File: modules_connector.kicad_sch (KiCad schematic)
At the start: 26 parts, among them J3 Conn_01x03, J4 Conn_01x03, J5 Conn_01x03, J9 Conn_01x04, K1 HE721A0500, K2 HE721A0500, Q1 BC847, Q2 BC847

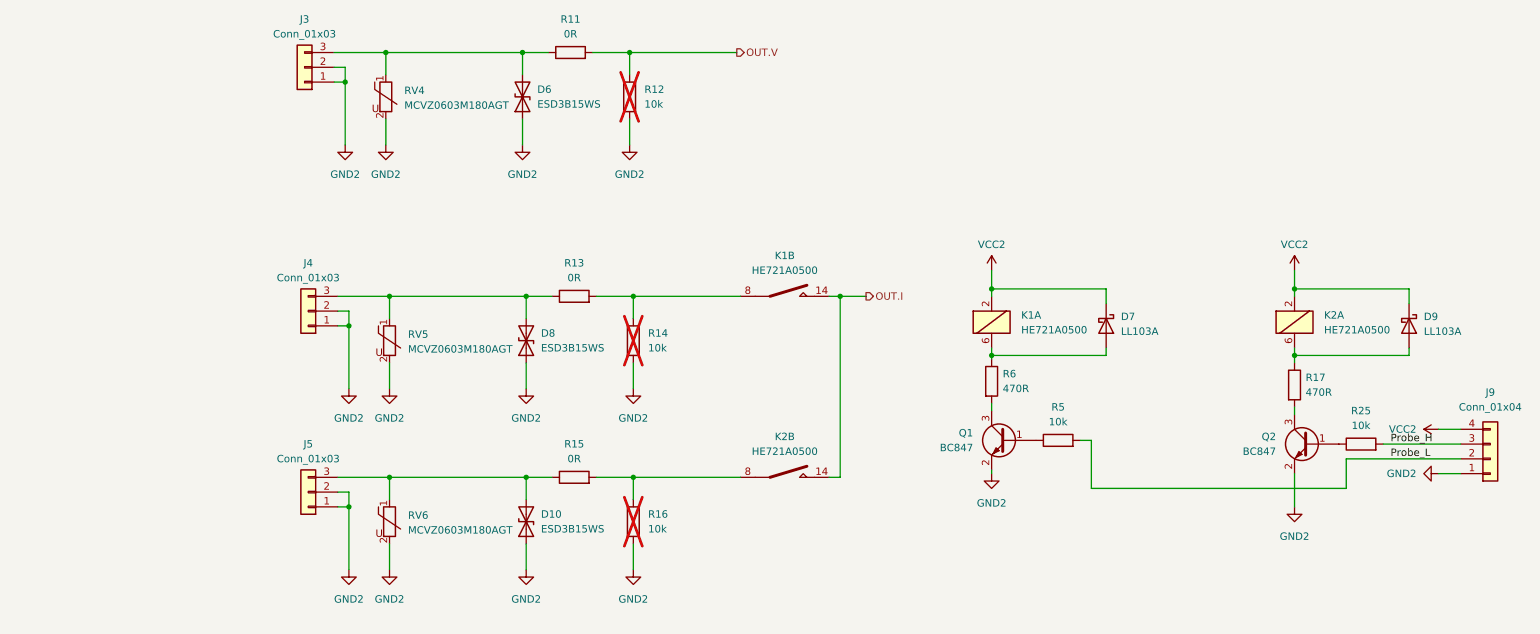
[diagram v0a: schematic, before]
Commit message: Redesign pcb
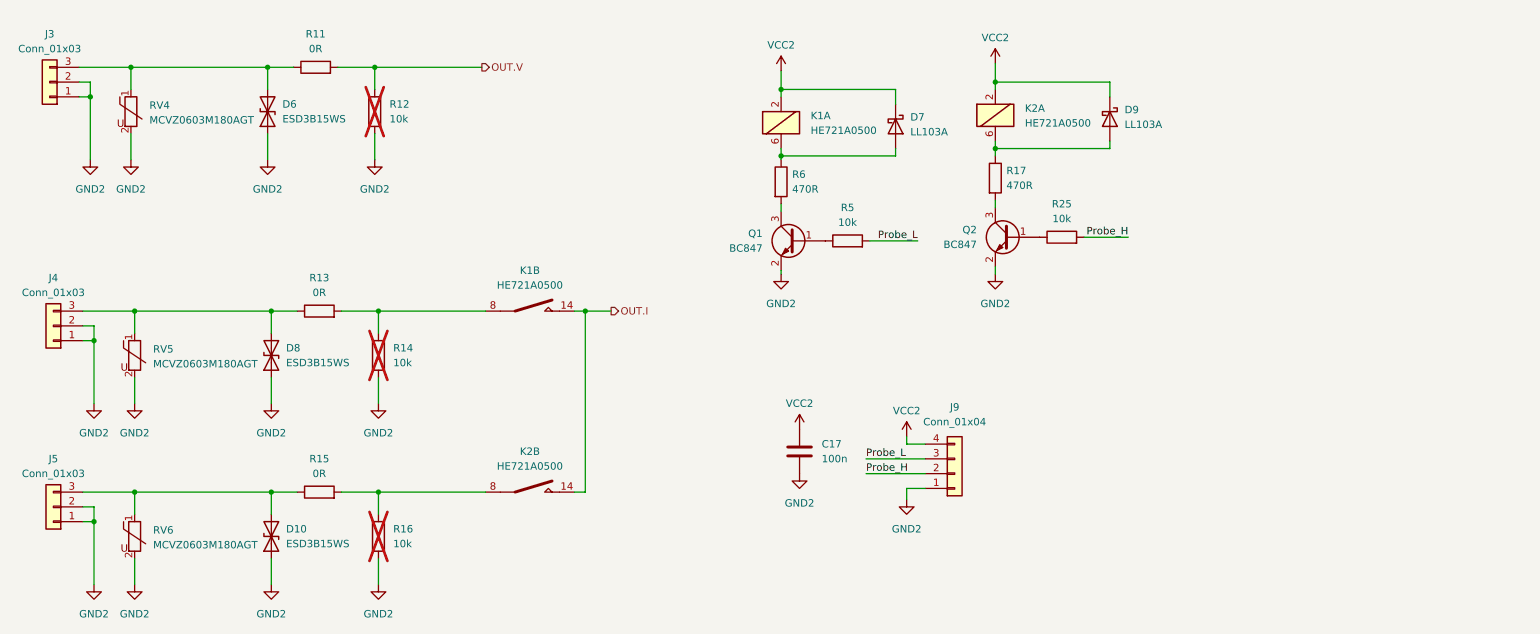
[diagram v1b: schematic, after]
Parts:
- added C17: 100n, Capacitor_SMD:C_0603_1608Metric, symbol Koszalix_Capacitors_Ceramic_Walsin_0603:CAP_100n_X7R
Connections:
- net GND2: now also C17.2
- net Probe_H: now also J9.2 (Pin_2); no longer J9.3 (Pin_3)
- net Probe_L: now also J9.3 (Pin_3); no longer J9.2 (Pin_2)
- net VCC2: now also C17.1
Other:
- moved on the sheet: D10, D6, D7, D8, D9, J3, J4, J5, J9, K1A, K1B, K2A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
